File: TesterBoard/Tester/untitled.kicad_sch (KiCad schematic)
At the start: 4 parts, among them U3 74LS04, U4 sn74ls32n, U5 CY62256-70PC, U6 28C256

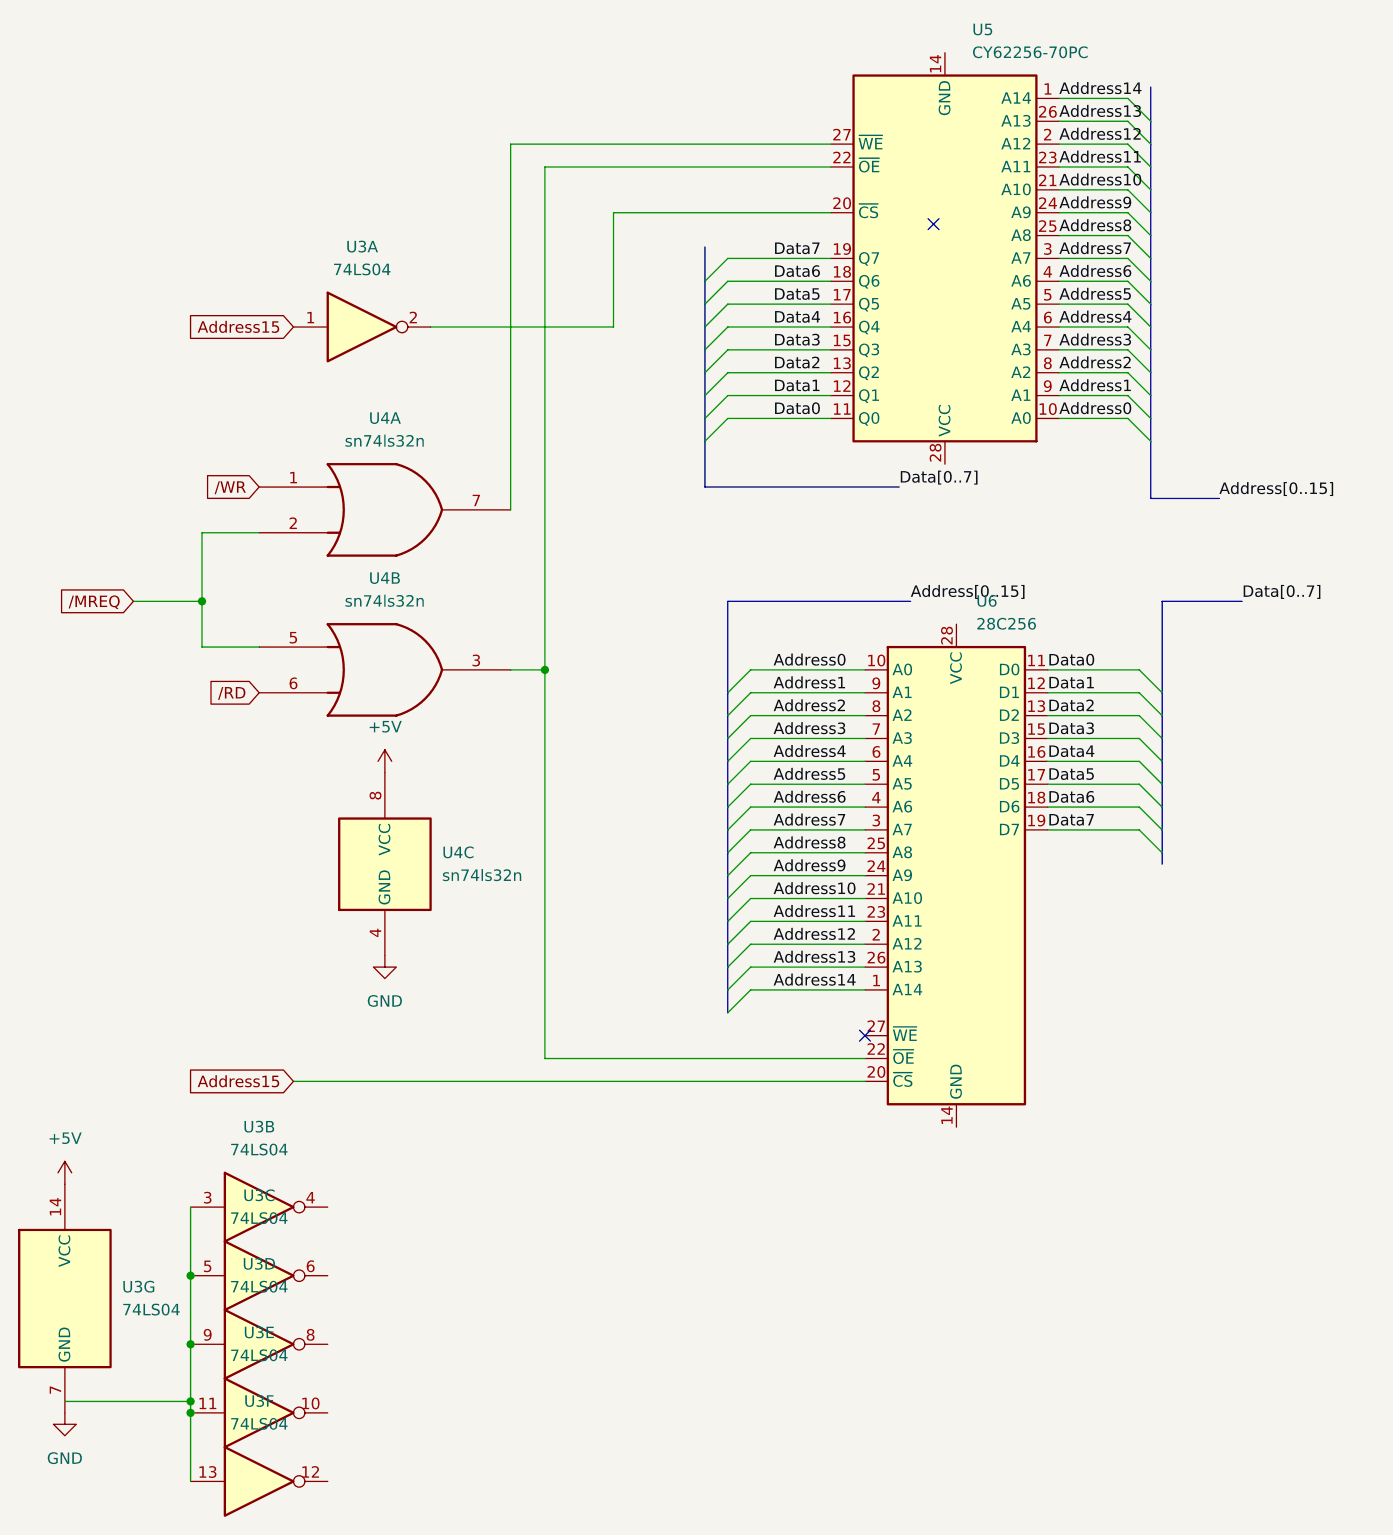
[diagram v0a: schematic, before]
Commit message: pcb stuff
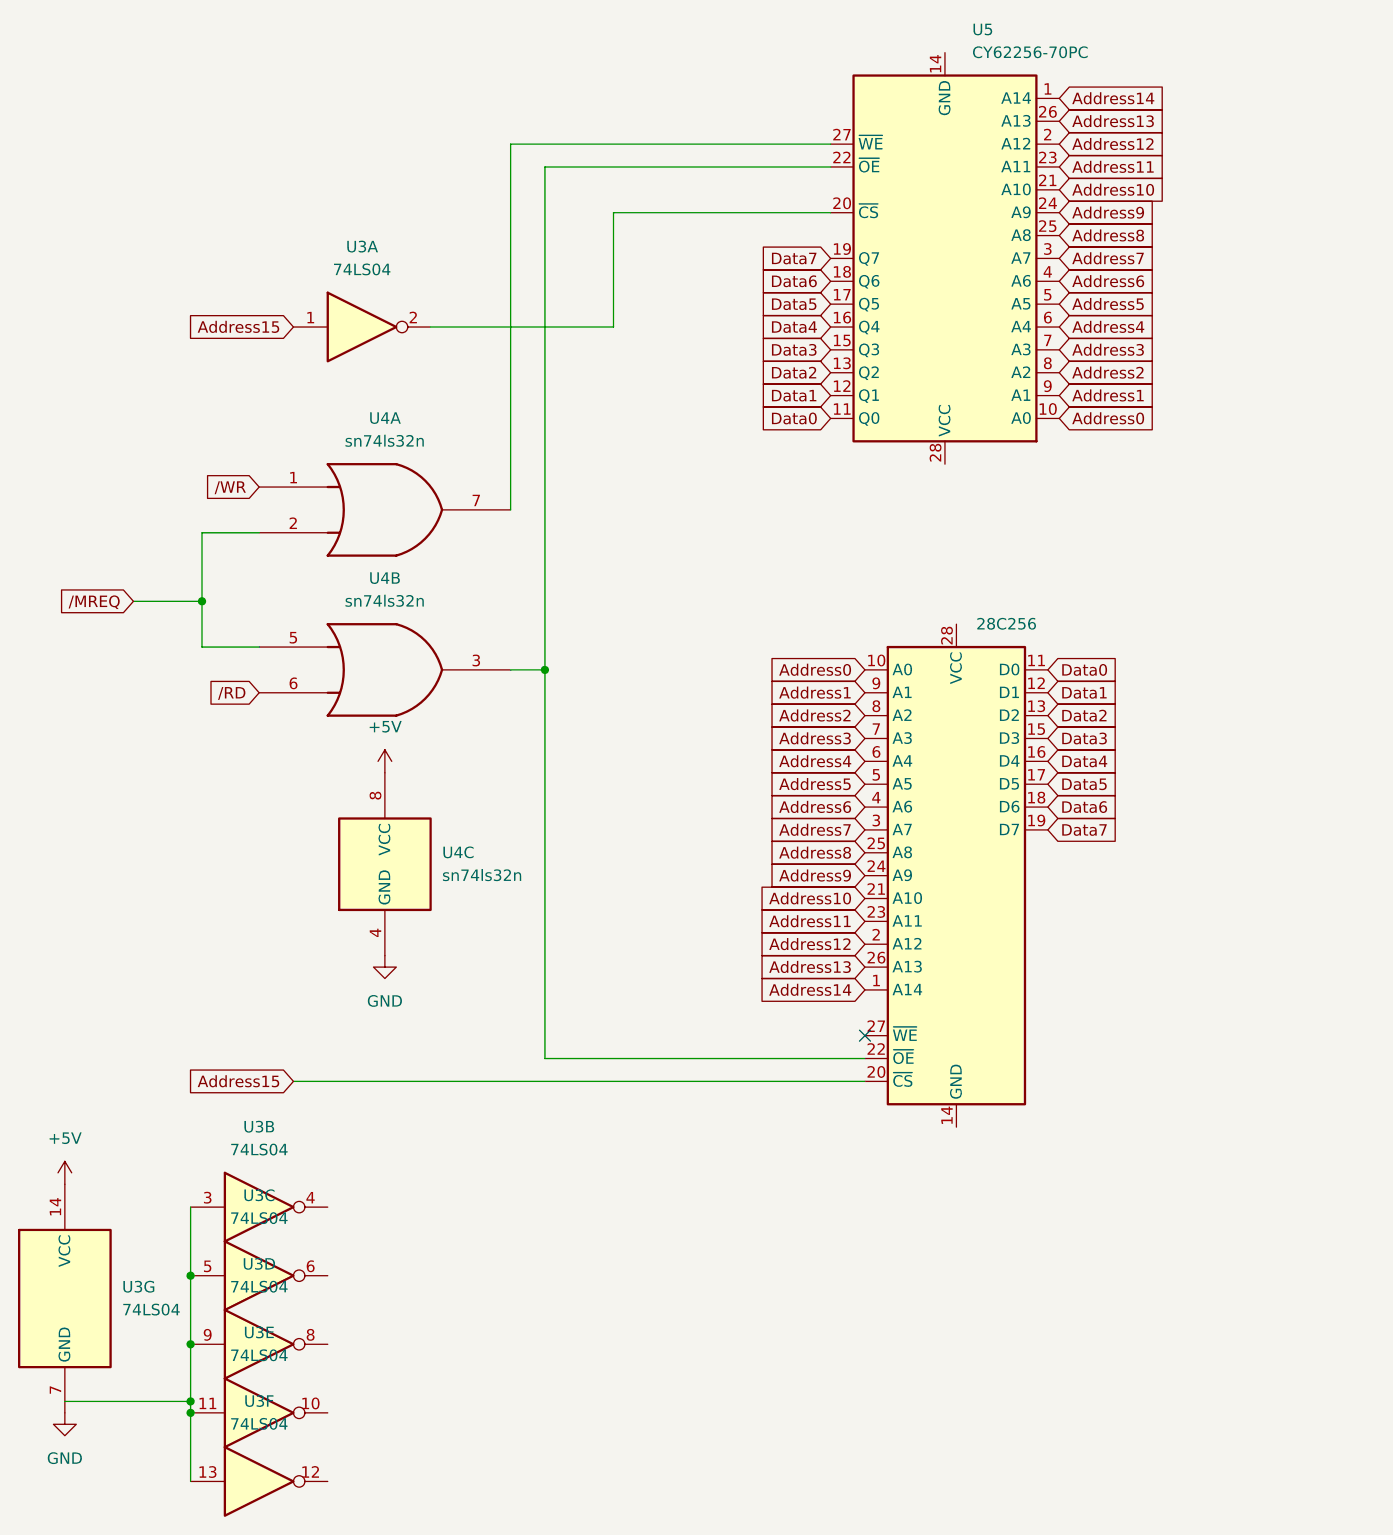
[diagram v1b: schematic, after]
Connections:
- no-connect marks 2 -> 1
